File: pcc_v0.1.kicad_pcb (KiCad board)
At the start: 2 copper layers, 53 parts, among them J1 Conn_01x04_Socket, J2 Conn_01x04_Socket, J4 Conn_02x14_Counter_Clockwise, J6 Conn_01x04_Socket, J7 Conn_01x04_Socket, J8 Conn_01x04_Socket, K2 CPC1706, K3 G7L-2A-X-L_DC12, U2 4N35, U3 4N35, U5 DMN63D8L-7, U8 SN65HVD230, U9 LM1117T-5.0

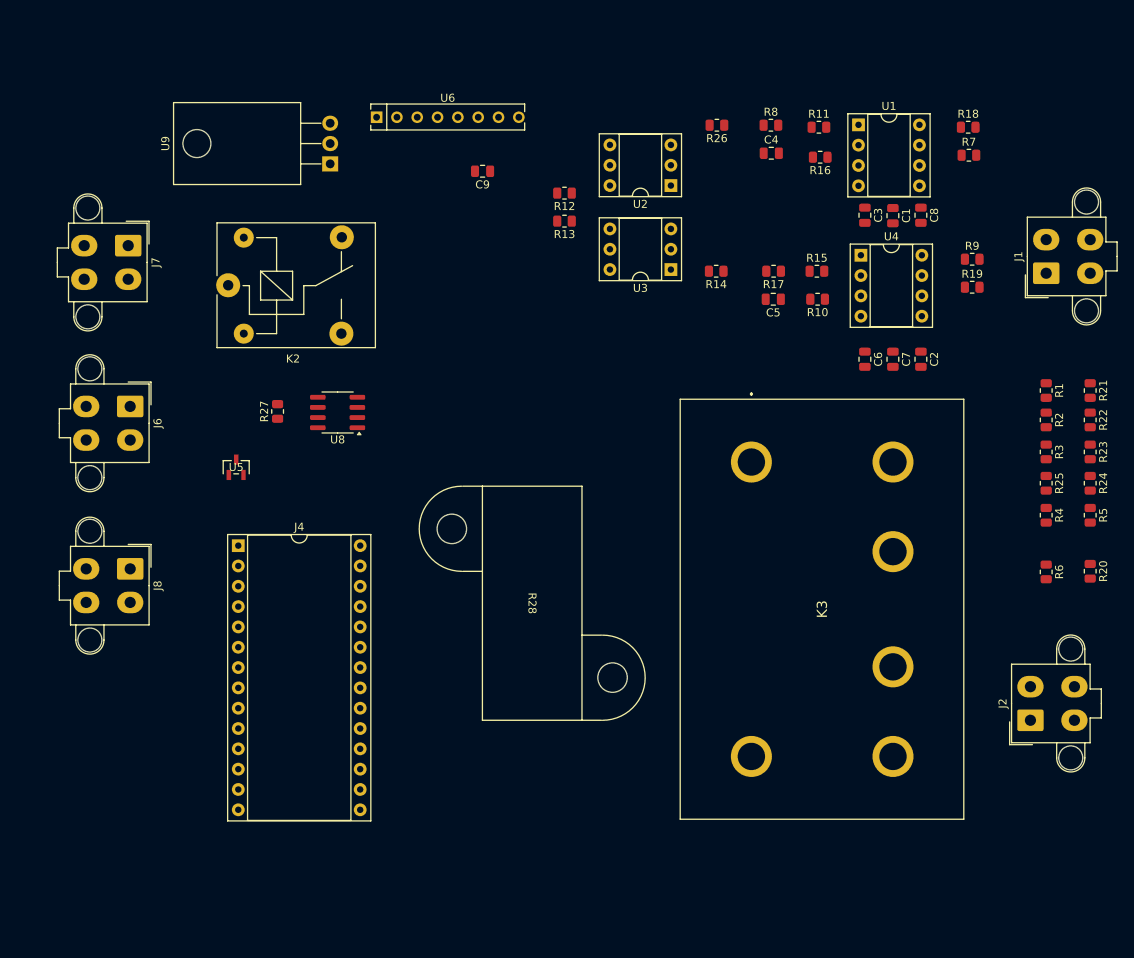
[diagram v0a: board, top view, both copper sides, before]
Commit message: routed pcb
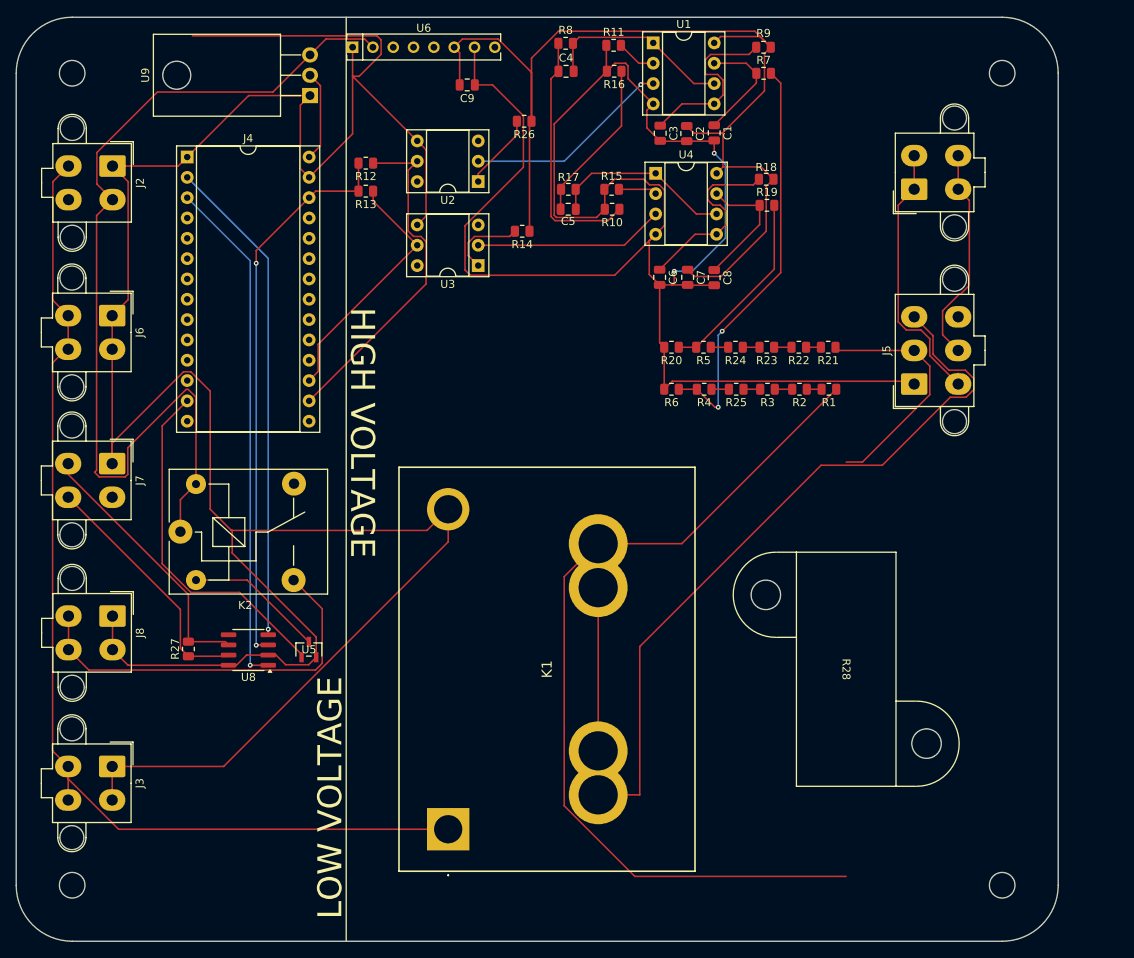
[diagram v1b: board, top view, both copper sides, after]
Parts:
- removed K3: G7L-2A-X-L_DC12, KiCad:G7L2AXLDC12
- added J3: Conn_01x04_Socket, Connector_Molex:Molex_Mini-Fit_Jr_5566-04A2_2x02_P4.20mm_Vertical, F.Cu at (101.2, 137.7)
- added J5: Conn_01x06_Socket, Connector_Molex:Molex_Mini-Fit_Jr_5566-06A2_2x03_P4.20mm_Vertical, F.Cu at (201.5, 89.8)
- added K1: G9KB-1A_DC12, precharge relay 2:G9KB1ADC12, F.Cu at (143.2, 145.5)
- added REF**: MountingHole_3.2mm_M3, MountingHole:MountingHole_3.2mm_M3, F.Cu at (96.2, 51.0)
- added REF**: MountingHole_3.2mm_M3, MountingHole:MountingHole_3.2mm_M3, F.Cu at (96.2, 152.5)
- added REF**: MountingHole_3.2mm_M3, MountingHole:MountingHole_3.2mm_M3, F.Cu at (212.5, 152.5)
- added REF**: MountingHole_3.2mm_M3, MountingHole:MountingHole_3.2mm_M3, F.Cu at (212.5, 51.0)
- R28: footprint footprints:RES_HSA25_TYCO_TYC -> precharge res:RES_HSA25_TYCO_TYC
- moved J2 134.0 mm to (101.3, 62.6), turned to -90 degrees
- moved R20 59.4 mm to (171.2, 85.2), turned to 180 degrees
- moved R5 52.7 mm to (175.2, 85.2), turned to 180 degrees
- moved R6 52.1 mm to (171.2, 90.5), turned to 180 degrees
- moved J4 49.0 mm to (110.6, 61.5)
- moved R24 47.5 mm to (179.2, 85.2), turned to 180 degrees
- moved R4 45.6 mm to (175.2, 90.5), turned to 180 degrees
- moved R23 42.5 mm to (183.1, 85.2), turned to 180 degrees
- moved C2 40.6 mm to (173.1, 58.5)
- moved R25 40.5 mm to (179.2, 90.5), turned to 180 degrees
- moved R28 40.1 mm to (193.0, 99.6)
- moved R22 37.5 mm to (187.1, 85.2), turned to 180 degrees
- moved R9 37.2 mm to (182.7, 47.8), turned to 180 degrees
- moved R3 35.7 mm to (183.2, 90.5), turned to 180 degrees
- moved R21 33.2 mm to (190.8, 85.2), turned to 180 degrees
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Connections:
- net IR-_12V renamed DISCHRG_COIL+
- J1 pad 1: GNDS -> DISCHRG_COM
- J1 pad 2: unconnected-(J1-Pin_2-Pad2) -> DISCHRG_COM
- J1 pad 3: Vin_TS -> DISCHRG_NO
- J1 pad 4: Vin_Accu -> DISCHRG_NO
- J4 pad 13: AIR+ -> IR+
- J4 pad 14: PRECHG -> unconnected-(J4-Pin_14-Pad14)
- J4 pad 26: unconnected-(J4-Pin_26-Pad26) -> +3.3V
- J7 pad 2: CANL -> unconnected-(J7-Pin_2-Pad2)
- J7 pad 3: CANH -> CANL
- J7 pad 4: unconnected-(J7-Pin_4-Pad4) -> CANH
- R21 pad 1: Vin_TS -> B+_out
- R28 pad 1: Net-(K3--_1) -> B+_out
- R28 pad 2: TS_in -> Vin_Accu
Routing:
- net GLV-: track 0.00 -> 330.2 mm
- net GNDS: track 0.00 -> 212.6 mm, vias 0 -> 2
- net +12P: track 0.00 -> 136.0 mm
- net DISCHRG_COIL+: track 0.00 -> 134.3 mm
- net +12V: track 0.00 -> 119.9 mm
- net Vin_Accu: track 0.00 -> 111.3 mm
- net B+_in: track 0.00 -> 92.2 mm
- net +3.3V: track 0.00 -> 70.2 mm, vias 0 -> 2
- net CANTX: track 0.00 -> 64.0 mm, vias 0 -> 1
- net CANRX: track 0.00 -> 61.4 mm, vias 0 -> 1
- net Net-(R4-Pad2): track 0.00 -> 51.3 mm, vias 0 -> 2
- net IR+_12V: track 0.00 -> 49.2 mm
- net IR+: track 0.00 -> 44.1 mm
- net Freq_Accumulator: track 0.00 -> 43.6 mm
- net DISCHRG_COM: track 0.00 -> 34.9 mm
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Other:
- board outline added: 130.2 x 115.5 mm
- board text added: "${REFERENCE}"
- board text added: "HIGH VOLTAGE"
- board text added: "LOW VOLTAGE"
